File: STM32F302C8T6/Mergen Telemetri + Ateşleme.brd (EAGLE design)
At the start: 49.7 x 87.5 mm, 99 parts, among them J2 U.FL, Q2 IRLML6344TRPBF, Q3 IRLML6344TRPBF, U1 AMS1117-3.3, U2 BMP280, U3 MPU-6050, U4 L86, U6 AMS1117-3.3, U7 AMS1117-3.3, U8 STM32F302C8T6, X1 JST-XH-04-PIN-LONG-PAD, Y2 ABM3B-26.000MHZ-10-1-U-T

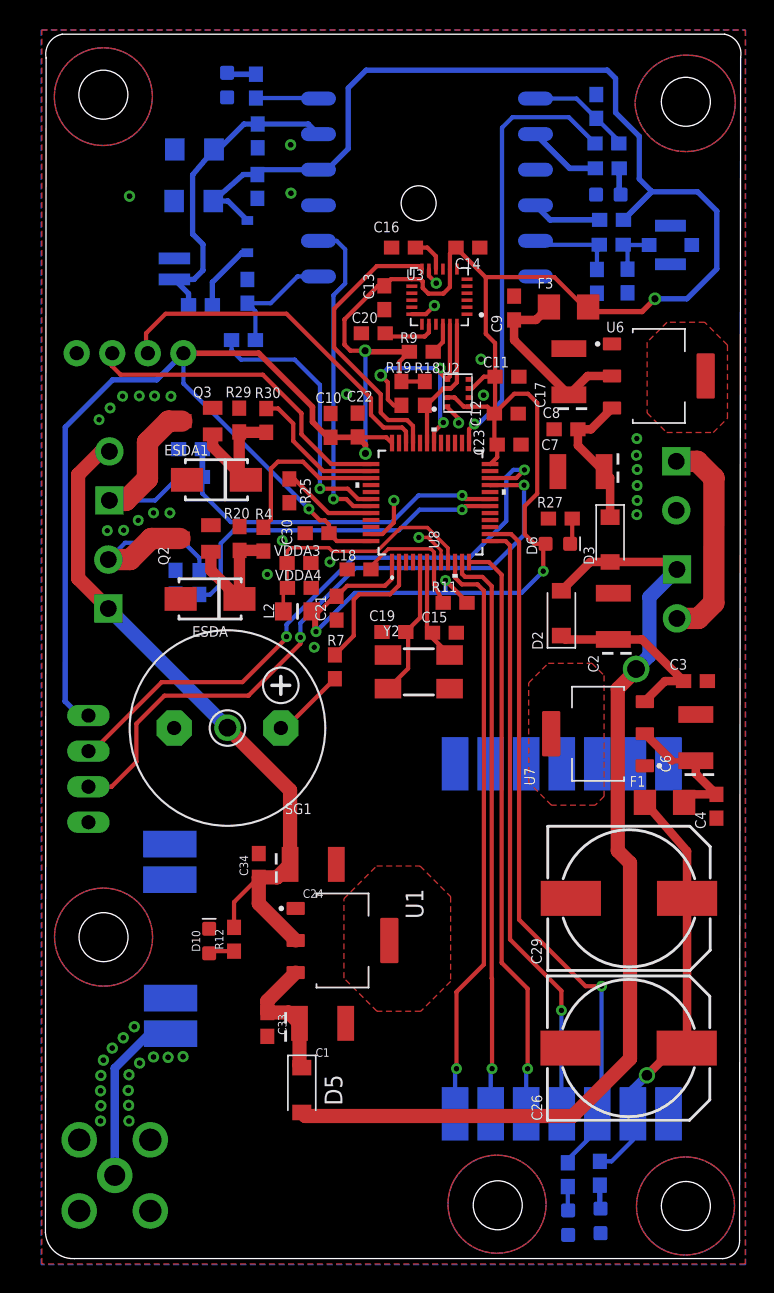
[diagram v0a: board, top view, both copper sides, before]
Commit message: Regulator name was changed as 5.0
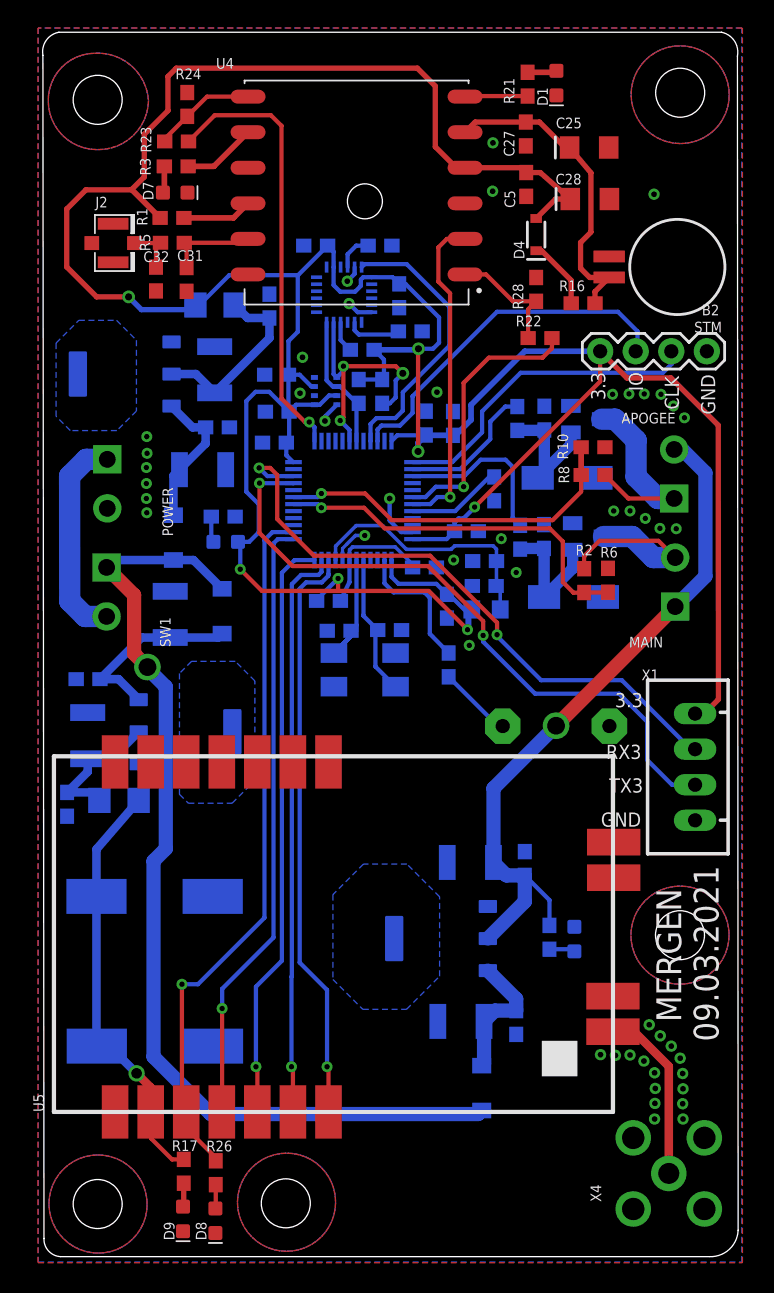
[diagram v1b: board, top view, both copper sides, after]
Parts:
- U1, U7: value AMS1117-3.3 -> AMS1117-5.0
- moved C4 46.4 mm to (2.34, 33.0), flipped to the bottom
- moved STM 45.0 mm to (48.0, 65.4), flipped to the top
- moved C6 43.4 mm to (3.81, 37.9), flipped to the bottom
- moved C3 43.4 mm to (3.84, 42.0), flipped to the bottom
- moved X1 43.3 mm to (47.2, 35.7), flipped to the top
- moved B2 40.8 mm to (45.9, 71.4), flipped to the top
- moved SW1 40.7 mm to (5.16, 49.9), flipped to the top
- moved POWER 40.6 mm to (5.21, 57.7), flipped to the top
- moved MAIN 40.5 mm to (45.8, 47.1), flipped to the top
- moved APOGEE 40.3 mm to (45.7, 54.9), flipped to the top
- moved J2 39.8 mm to (5.62, 73.1), flipped to the top
- moved X4 39.6 mm to (45.3, 6.65), flipped to the top
- moved F1 39.0 mm to (6.05, 33.3), flipped to the bottom
- moved U6 38.2 mm to (6.45, 63.8), flipped to the bottom
- moved C29 33.9 mm to (8.59, 26.4), flipped to the bottom
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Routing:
- added copper zone on layer 16, net HT
- added copper zone on layer 16, net HT2
- added copper zone on layer 16, net HT3
- removed copper zone on layer 1, net HT
- removed copper zone on layer 1, net HT2
- removed copper zone on layer 1, net HT3
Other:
- outline, holes or cut-outs redrawn
- board text added: "3.3"
- board text added: "CLK"
- board text added: "GND"
- board text added: "IO"
- board text added: "RX3"
- board text added: "TX3"
